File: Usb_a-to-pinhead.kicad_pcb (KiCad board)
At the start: 2 copper layers, 34.7 x 18 mm, 4 parts, among them J1 USB_A, J2 Conn_01x02_Pin

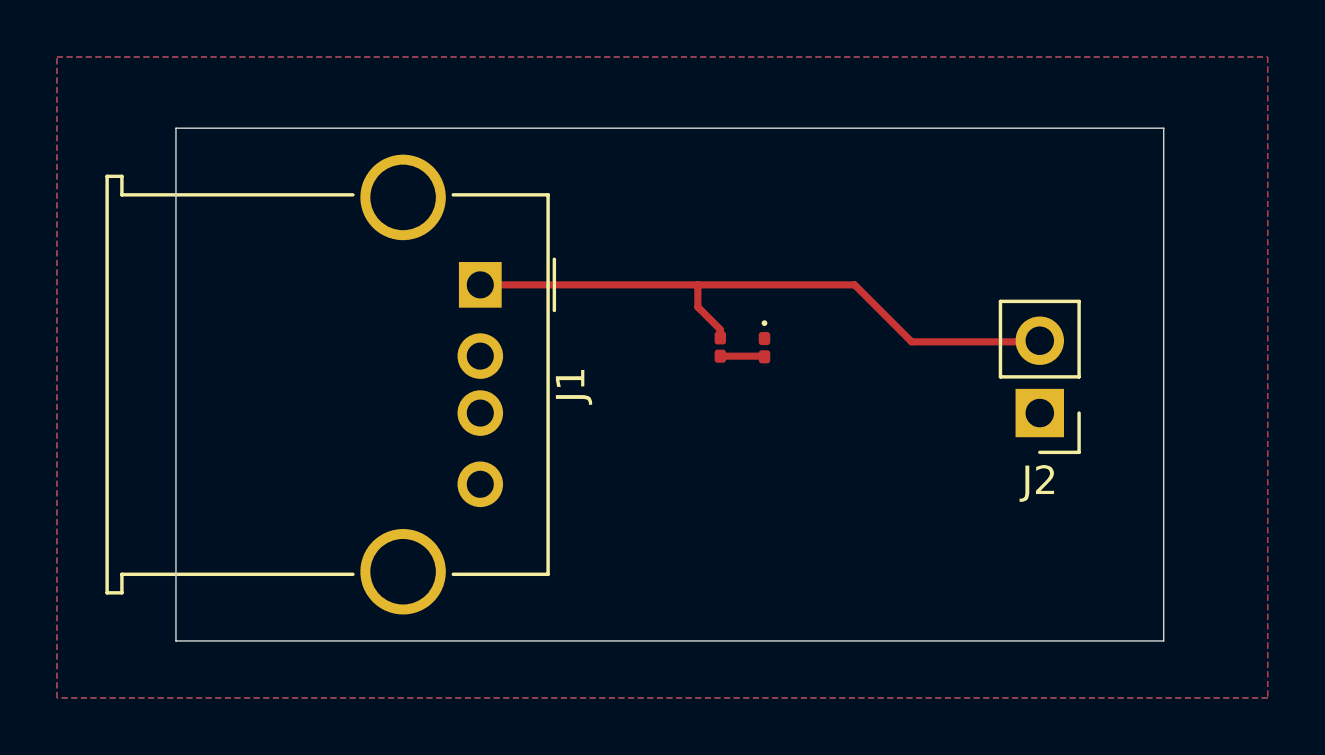
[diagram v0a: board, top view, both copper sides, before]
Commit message: 2026-03-9 | So-Mo
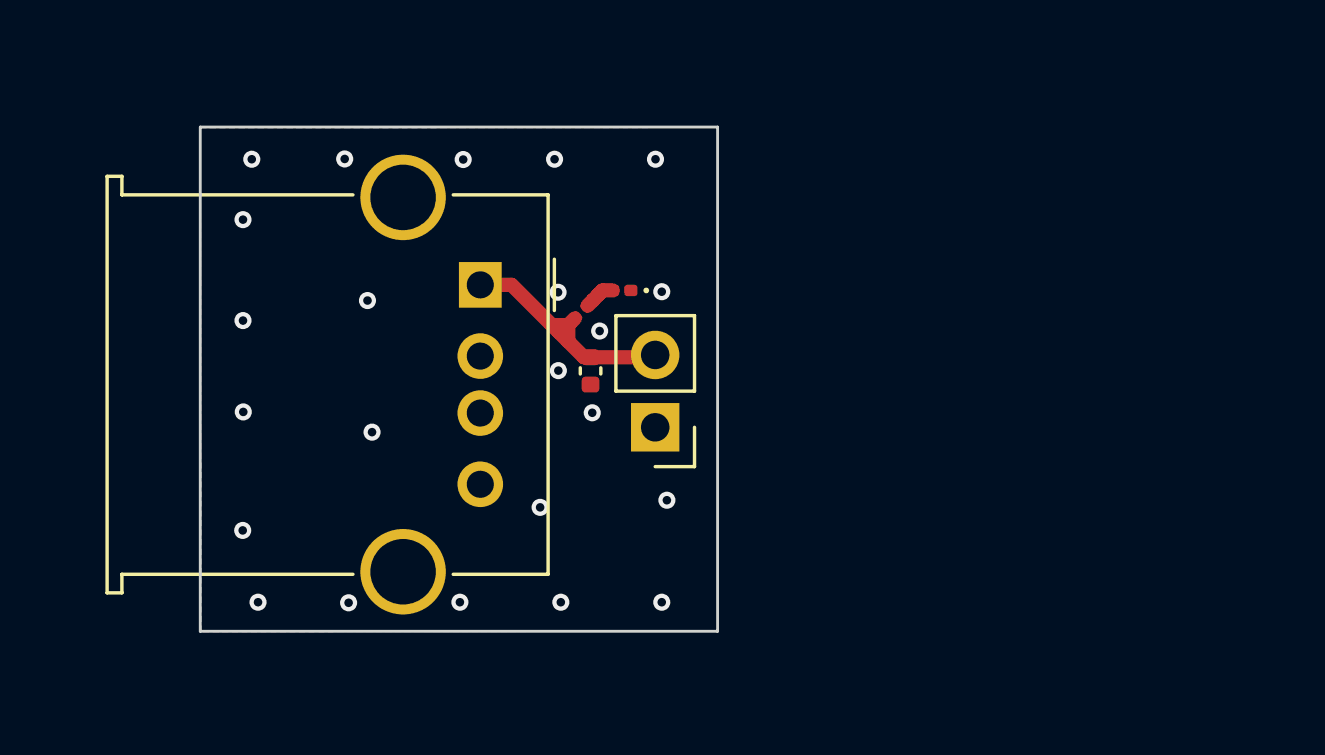
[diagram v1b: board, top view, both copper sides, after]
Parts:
- added C1: 100nF, Capacitor_SMD:C_0402_1005Metric, F.Cu at (128.7, 86.0)
- moved J2 13.5 mm to (131.0, 88.0)
- moved D1 5.40 mm to (129.8, 83.2), turned to 180 degrees
- moved R1 5.03 mm to (128.4, 84.0), turned to 45 degrees
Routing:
- net +5V: track 23.4 -> 9.22 mm
- net (no net): vias 0 -> 23
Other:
- board size 34.7 x 18 mm -> 18.2 x 17.7 mm
